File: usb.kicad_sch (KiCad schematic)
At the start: 130 parts, among them J3 USB4105-GF-A, J4 WE_632723300011_alt_symbol, U10 TUSB1046-DCI, U11 TPD4E05U06QDQARQ1, U12 AP22615, U13 TPD4E05U06QDQARQ1, U14 TPD4E05U06QDQARQ1, U15 TPD4E05U06QDQARQ1, U16 TPD4E05U06QDQARQ1, U5 FT230XQ-R, U6 TPS65988, U7 W25Q80DVUXIE_TR, U8 NCP730BMT330TBG, U9 AP22615

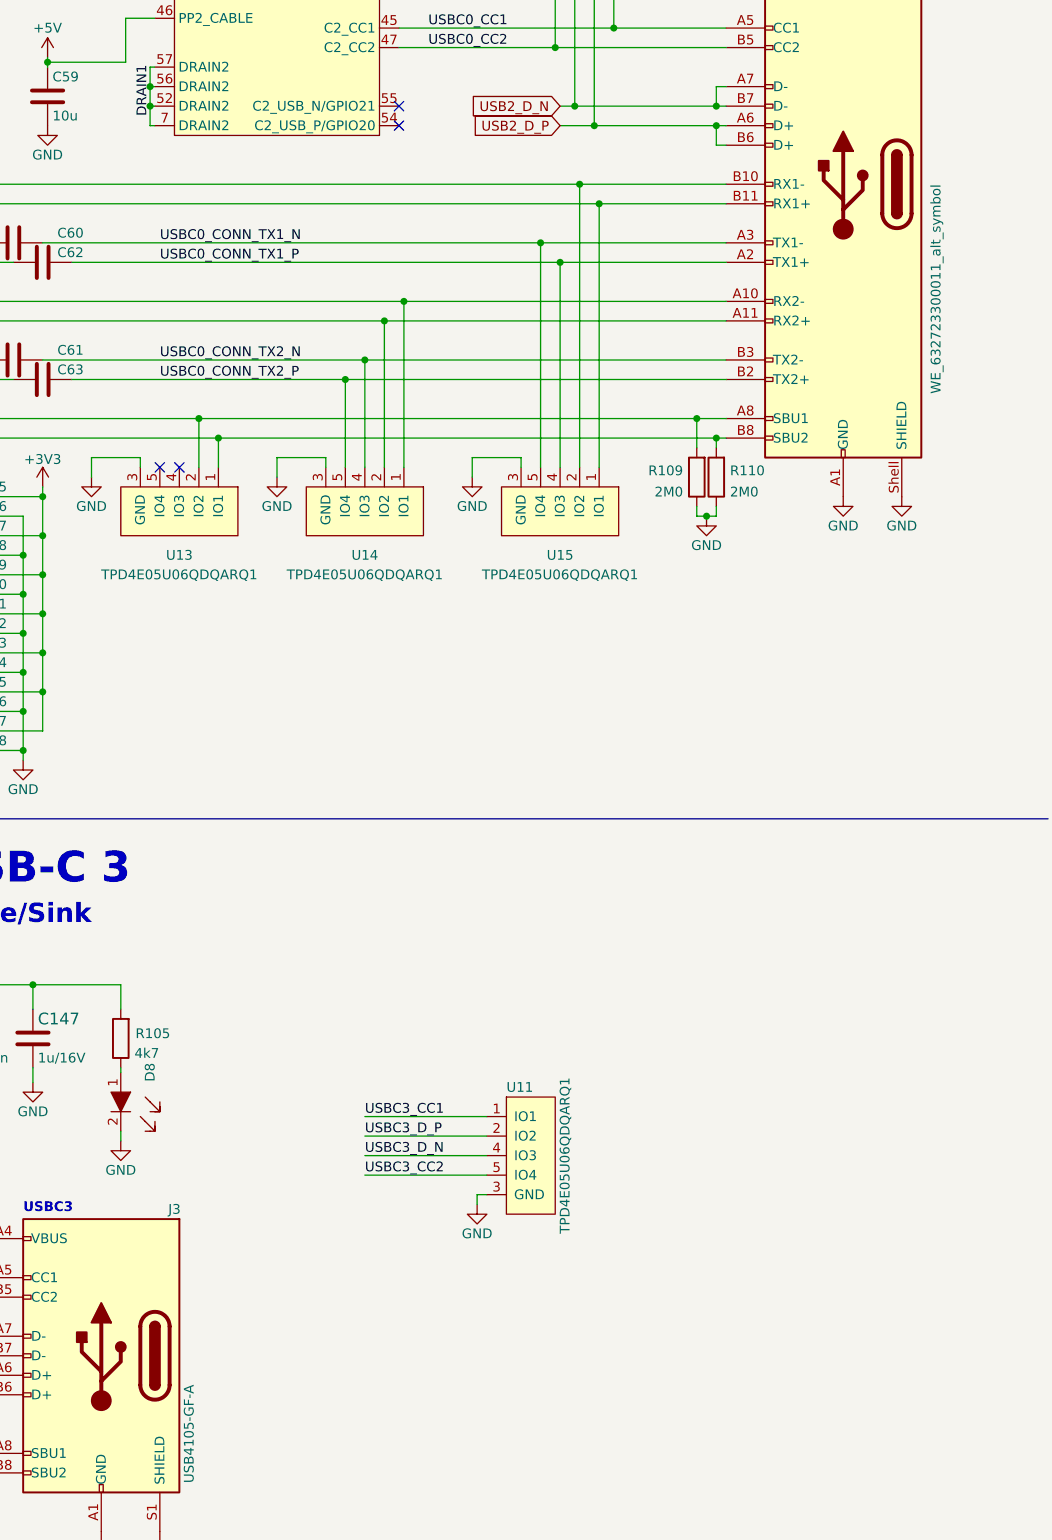
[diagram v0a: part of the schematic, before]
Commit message: Simplification continues
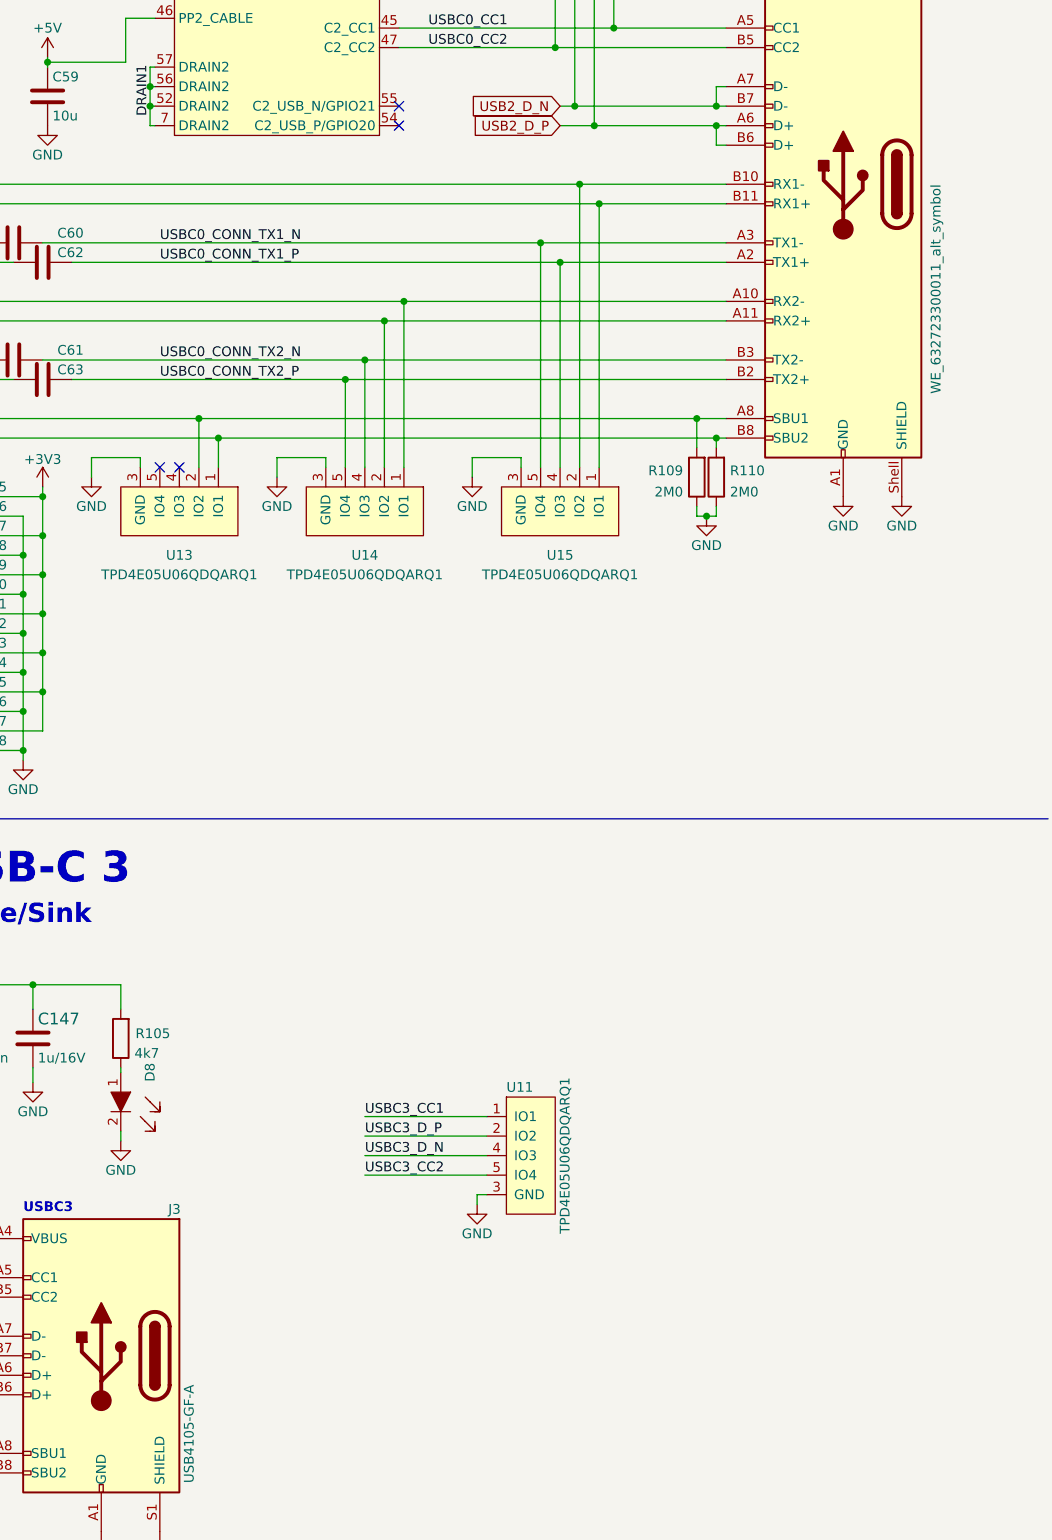
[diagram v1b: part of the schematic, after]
